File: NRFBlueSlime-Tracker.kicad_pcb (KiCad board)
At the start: 2 copper layers, 30 x 31.8 mm, 29 parts, among them J1 532610271, J2 Conn_01x06_Pin, SW1 TS-1088-AR02016, U1 ISP1507-AX-ST, U2 ICM-42688-P, U3 LIS2MDL, U4 ME6211C33R5G, U5 SRV05-4, X1 S2D32.768KB20F30T

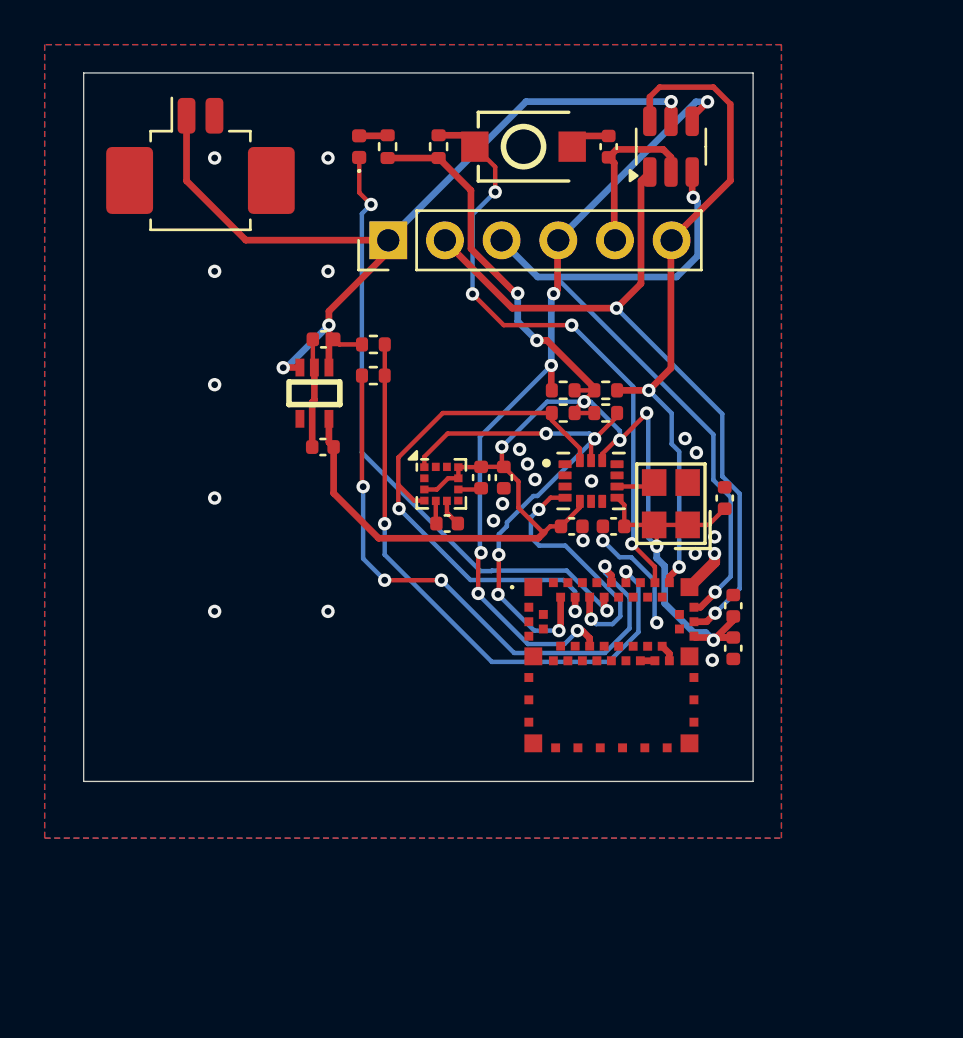
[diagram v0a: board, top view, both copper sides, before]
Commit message: mdbt42
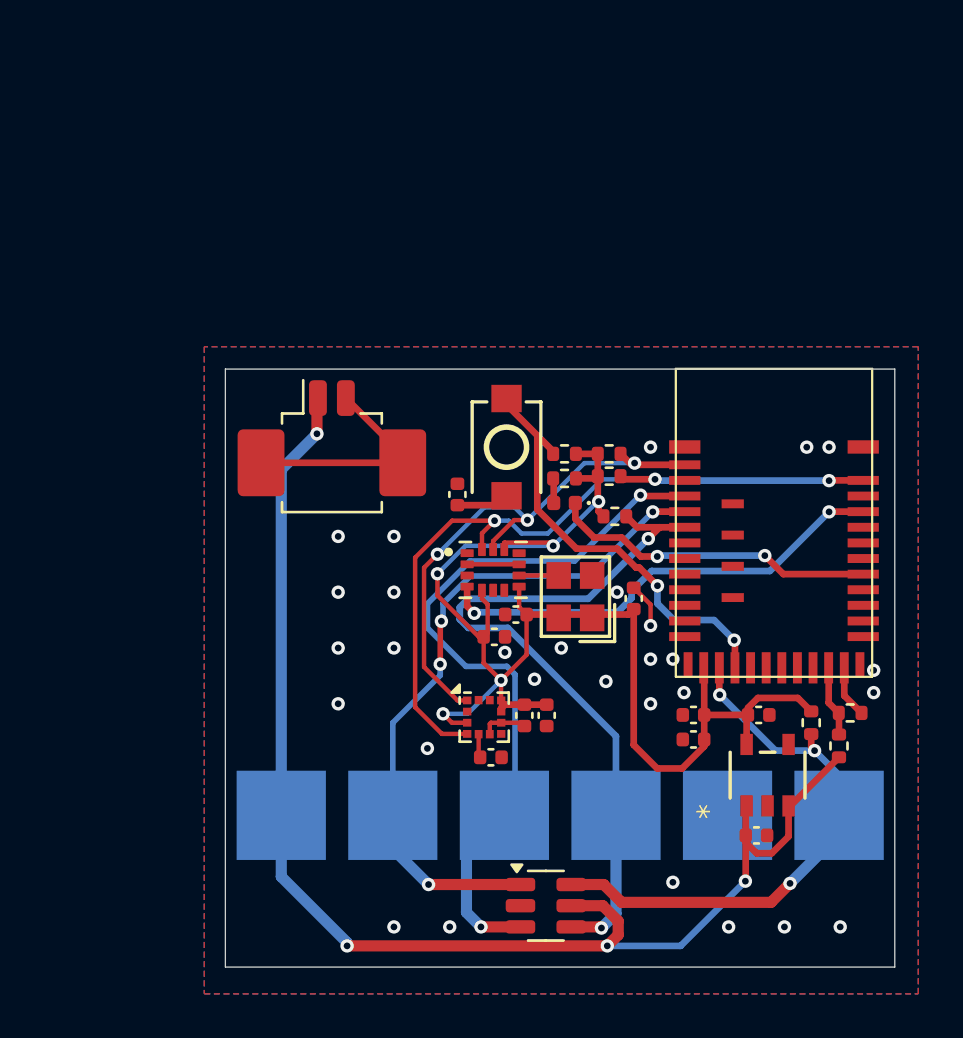
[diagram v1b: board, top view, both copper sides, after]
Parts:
- added J3: Conn_01x01, TestPoint:TestPoint_Pad_4.0x4.0mm, B.Cu at (129.9, 95.5)
- added J4: Conn_01x01, TestPoint:TestPoint_Pad_4.0x4.0mm, B.Cu at (134.9, 95.5)
- added J5: Conn_01x01, TestPoint:TestPoint_Pad_4.0x4.0mm, B.Cu at (139.9, 95.5)
- added J6: Conn_01x01, TestPoint:TestPoint_Pad_4.0x4.0mm, B.Cu at (144.9, 95.5)
- added J7: Conn_01x01, TestPoint:TestPoint_Pad_4.0x4.0mm, B.Cu at (149.9, 95.5)
- J2: value Conn_01x06_Pin -> Conn_01x01; footprint Connector_PinHeader_2.54mm:PinHeader_1x06_P2.54mm_Vertical -> TestPoint:TestPoint_Pad_4.0x4.0mm; moved to B.Cu
- U1: value ISP1507-AX-ST -> MDBT42-512KV2; footprint ISP1507-AX-ST:ISP1507AXST -> MDBT42:MDBT42
- U4: value ME6211C33R5G -> RT9080-33GJ5; footprint nrfslime:SOT-353_L2.1-W1.3-P0.65-LS2.3-BL -> RT9080:TSOT-23-5_RIT
- moved U5 34.5 mm to (136.8, 99.5), turned to 0 degrees
- moved C6 29.5 mm to (146.2, 96.4), turned to 0 degrees
- moved R3 27.6 mm to (149.9, 92.4), turned to 90 degrees
- moved U4 26.6 mm to (146.7, 93.7), turned to 90 degrees
- moved J2 26.2 mm to (124.9, 95.5), turned to 180 degrees
- moved R8 26.2 mm to (150.4, 90.9), turned to 0 degrees
- moved C7 22.9 mm to (146.3, 91.0), turned to 0 degrees
- moved LED1 18.4 mm to (137.6, 81.5), turned to 180 degrees
- moved R4 17.5 mm to (148.7, 91.3), turned to -90 degrees
- moved C11 17.0 mm to (132.8, 81.1), turned to 90 degrees
- moved R2 16.8 mm to (137.6, 80.4), turned to 180 degrees
- moved U1 15.2 mm to (147.0, 75.5)
- moved R1 14.9 mm to (137.6, 79.3), turned to 180 degrees
- moved J1 14.0 mm to (127.2, 79.2)
- moved SW1 13.5 mm to (135.0, 79.0), turned to -90 degrees
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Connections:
- U1 pad 10: GND -> unconnected-(U1-P0.13-Pad10)
- U1 pad 12: GND -> unconnected-(U1-P0.10-Pad12)
- U1 pad 13: RST -> unconnected-(U1-P0.09-Pad13)
- U1 pad 15: unconnected-(U1-P0_20/TRACE_CLK-Pad15) -> +3V3
- U1 pad 16: GND -> DOCK
- U1 pad 17: unconnected-(U1-P0_22-Pad17) -> KEY
- U1 pad 18: GND -> unconnected-(U1-P0.07-Pad18)
- U1 pad 2: unconnected-(U1-P0_09/NFC1-Pad2) -> SCL
- U1 pad 20: Net-(U1-OUT_ANT) -> unconnected-(U1-P0.00/XL1-Pad20)
- U1 pad 21: GND -> unconnected-(U1-P0.01/XL2-Pad21)
- U1 pad 22: Net-(U1-OUT_ANT) -> unconnected-(U1-P0.04-Pad22)
- U1 pad 23: GND -> BATLVL
- U1 pad 24: GND -> ADC_EN
- U1 pad 26: +3V3 -> unconnected-(U1-DCC-Pad26)
- U1 pad 28: SWD -> unconnected-(U1-P0.31-Pad28)
- U1 pad 30: SWC -> LED
- U1 pad 31: GND -> unconnected-(U1-P0.30-Pad31)
- U1 pad 32: DOCK -> unconnected-(U1-P0.29-Pad32)
- U1 pad 34: KEY -> INT
- U1 pad 36: unconnected-(U1-P0_05/AIN3-Pad36) -> SDA
- U1 pad 37: unconnected-(U1-P0_15/TRACE_DATA2-Pad37) -> GND
- U1 pad 38: BATLVL -> unconnected-(U1-P0.24-Pad38)
- U1 pad 4: unconnected-(U1-P0_10/NFC2-Pad4) -> SWC
- U1 pad 40: ADC_EN -> unconnected-(U1-P0.16-Pad40)
- U1 pad 41: LED -> unconnected-(U1-P0.14-Pad41)
- U1 pad 5: unconnected-(U1-P0_14/TRACE_DATA3-Pad5) -> SWD
- U1 pad 6: unconnected-(U1-P0_26-Pad6) -> RST
- U1 pad 7: GND -> unconnected-(U1-P0.18-Pad7)
- U1 pad 8: GND -> unconnected-(U1-P0.17-Pad8)
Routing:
- net ADC_EN: track 26.5 -> 2.34 mm, vias 4 -> 0
- net BATLVL: track 26.8 -> 3.18 mm, vias 2 -> 0
- net +BATT: track 41.8 -> 59.9 mm, vias 3 -> 4
- net +3V3: track 76.9 -> 62.7 mm, vias 8 -> 5
- net LED: track 28.2 -> 14.7 mm
- net SDA: track 25.1 -> 34.7 mm, vias 2 -> 3
- net INT: track 11.2 -> 20.8 mm
- net KEY: track 27.4 -> 19.6 mm, vias 4 -> 2
- net GND: track 22.5 -> 16.7 mm, vias 23 -> 29
- net DOCK: track 30.3 -> 25.1 mm, vias 2 -> 3
- net SWD: track 33.3 -> 30.8 mm, vias 2 -> 4
- net RST: track 35.6 -> 33.2 mm, vias 6 -> 2
- net SWC: track 32.6 -> 33.7 mm
- net SCL: track 25.0 -> 24.2 mm, vias 5 -> 3
- net Net-(U1-OUT_ANT): track 0.65 -> 0.00 mm
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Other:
- board size 30 x 31.8 mm -> 30 x 26.8 mm
